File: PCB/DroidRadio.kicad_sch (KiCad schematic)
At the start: 31 parts, among them T1 MABA-007159, U1 LTC5599IUF, U2 ADF4351

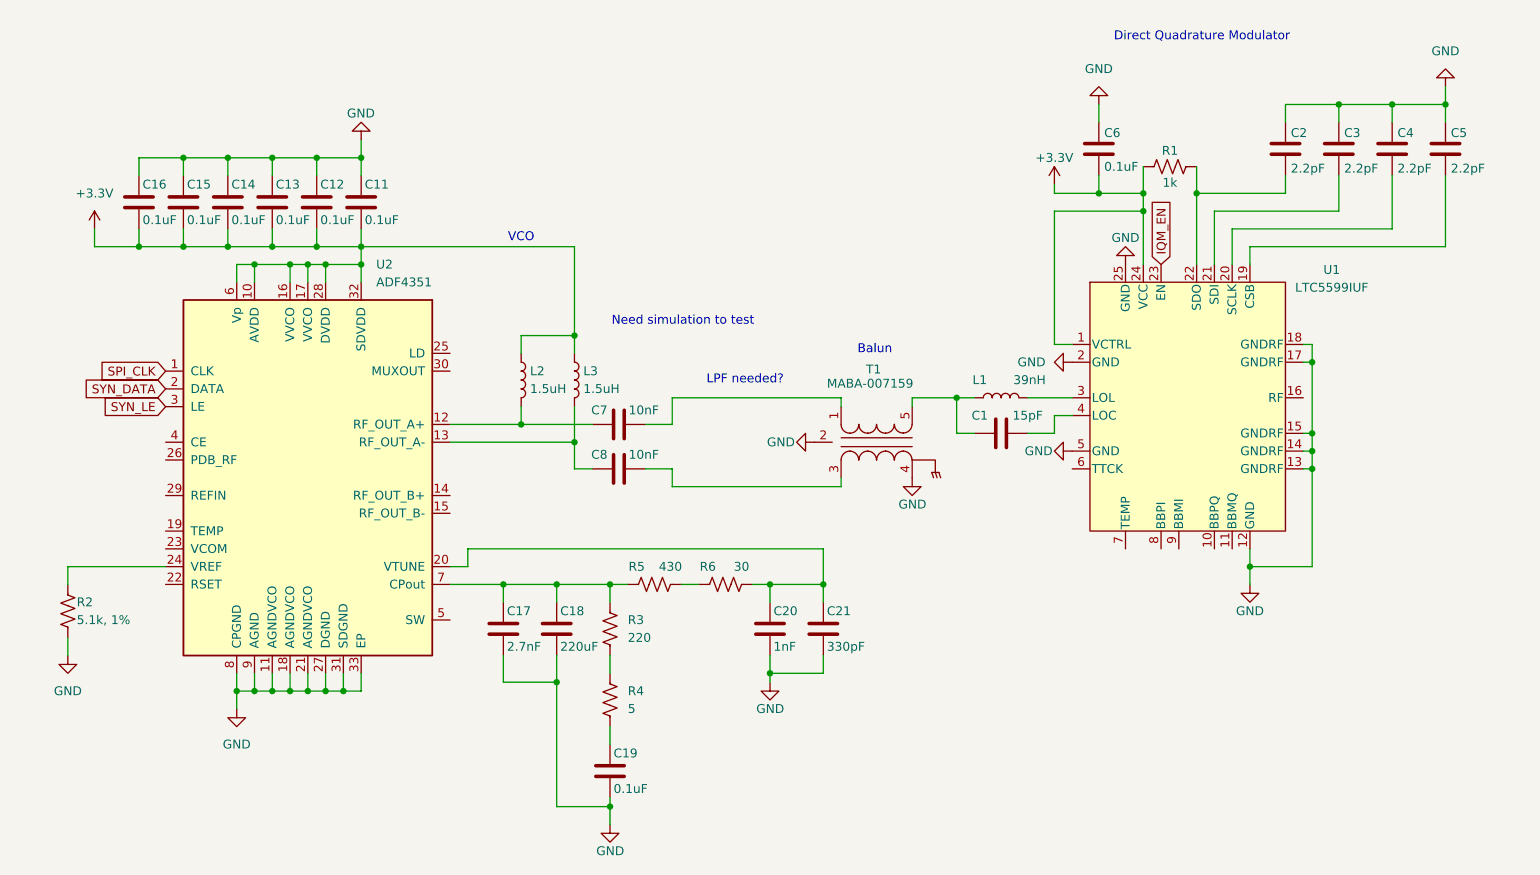
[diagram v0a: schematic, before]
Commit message: new file:   .gitignore 	modified:   PCB/DroidRadio.kicad_pro 	modified:   PCB/DroidRadio.kicad_sch 	new file:   PCB/Processors.kicad_sch 	new file:   PCB/Transmitter.kicad_sch 	deleted:    PCB/_autosave-Transmitter.kicad_sch 	new file:   PCB/~DroidRadio.kicad_pro.lck
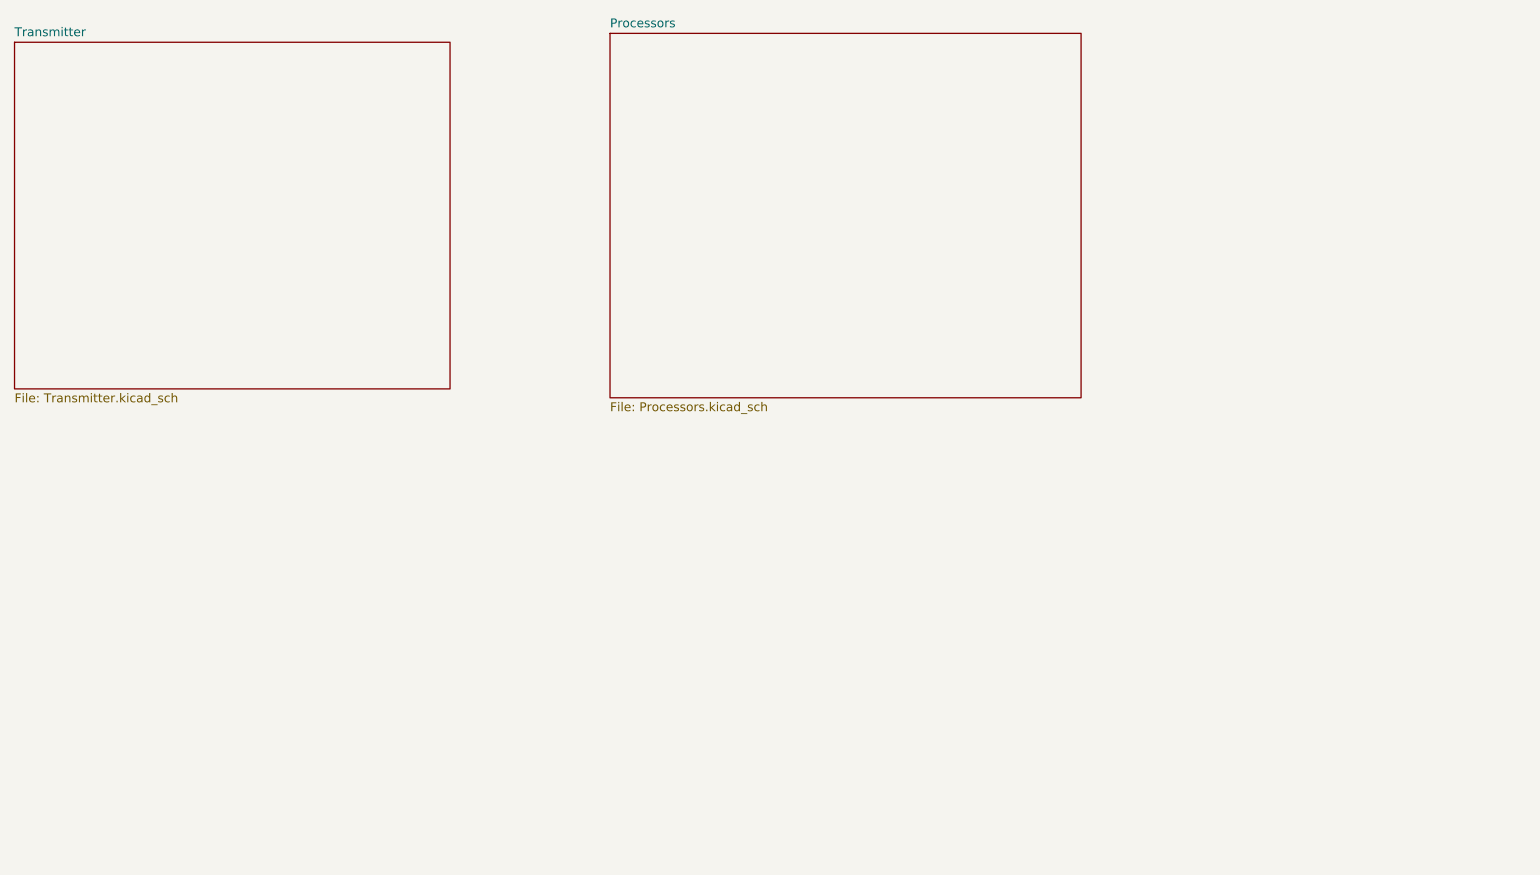
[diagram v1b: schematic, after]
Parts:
- removed C1: 15pF, symbol Device:C
- removed C11, C12, C13, C14, C15, C16, C19, C6: 0.1uF, symbol Device:C
- removed C17: 2.7nF, symbol Device:C
- removed C18: 220uF, symbol Device:C
- removed C2, C3, C4, C5: 2.2pF, symbol Device:C
- removed C20: 1nF, symbol Device:C
- removed C21: 330pF, symbol Device:C
- removed C7, C8: 10nF, symbol Device:C
- removed L1: 39nH, symbol Device:L
- removed L2, L3: 1.5uH, symbol Device:L
- removed R1: 1k, symbol Device:R_US
- removed R2: 5.1k, 1%, symbol Device:R_US
- removed R3: 220, symbol Device:R_US
- removed R4: 5, symbol Device:R_US
- removed R5: 430, symbol Device:R_US
- removed R6: 30, symbol Device:R_US
- removed T1: MABA-007159, MABA-007159-000000_MCM, symbol DroidRadio:MABA-007159
- removed U1: LTC5599IUF, DroidRadio:QFN-24_UF_LIT, symbol DroidRadio:LTC5599IUF
- removed U2: ADF4351, Package_CSP:LFCSP-32-1EP_5x5mm_P0.5mm_EP3.25x3.25mm, symbol Timer_PLL:ADF4351
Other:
- added sheet Processors (Processors.kicad_sch)
- added sheet Transmitter (Transmitter.kicad_sch)
- note removed: "Balun"
- note removed: "Direct Quadrature Modulator"
- note removed: "LPF needed?"
- note removed: "Need simulation to test"
- note removed: "VCO"

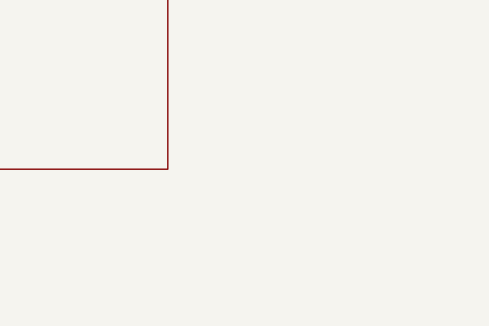
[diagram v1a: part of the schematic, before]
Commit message: new file:   Datasheet/HMC849A_RF_Switch_SPDT.pdf 	new file:   Datasheet/TG2016SMN_26MHz_MCGNNM_Oscillator.pdf 	modified:   PCB/DroidRadio.kicad_pro 	modified:   PCB/DroidRadio.kicad_sch 	modified:   PCB/Processors.kicad_sch 	modified:   PCB/Simulation/Transmitter_Side.pll 	modified:   PCB/Transmitter.kicad_sch 	deleted:    PCB/~DroidRadio.kicad_pro.lck
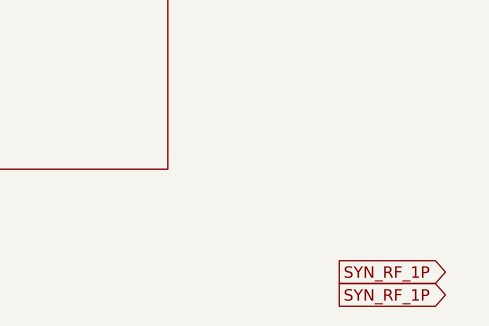
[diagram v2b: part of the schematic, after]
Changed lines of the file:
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@@
 	(generator_version "10.0")
 	(paper "A4")
+	(global_label "SYN_RF_1P"
+		(shape output)
+		(at 205.74 96.52 0)
+		(fields_autoplaced yes)
+		(effects
+			(font
+				(size 1.27 1.27)
+			)
+			(justify left)
+		)
+		(property "Intersheetrefs" "${INTERSHEET_REFS}"
+			(at 219.1271 96.52 0)
+			(hide yes)
+			(show_name no)
+			(do_not_autoplace no)
+			(effects
+				(font
+					(size 1.27 1.27)
+				)
+				(justify left)
+			)
+		)
+	)
+	(global_label "SYN_RF_1P"
+		(shape output)
+		(at 205.74 99.06 0)
+		(fields_autoplaced yes)
+		(effects
+			(font
+				(size 1.27 1.27)
+			)
+			(justify left)
+		)
+		(property "Intersheetrefs" "${INTERSHEET_REFS}"
+			(at 219.1271 99.06 0)
+			(hide yes)
+			(show_name no)
+			(do_not_autoplace no)
+			(effects
+				(font
+					(size 1.27 1.27)
+				)
+				(justify left)
+			)
+		)
+	)
 	(sheet
 		(at 34.29 34.29)

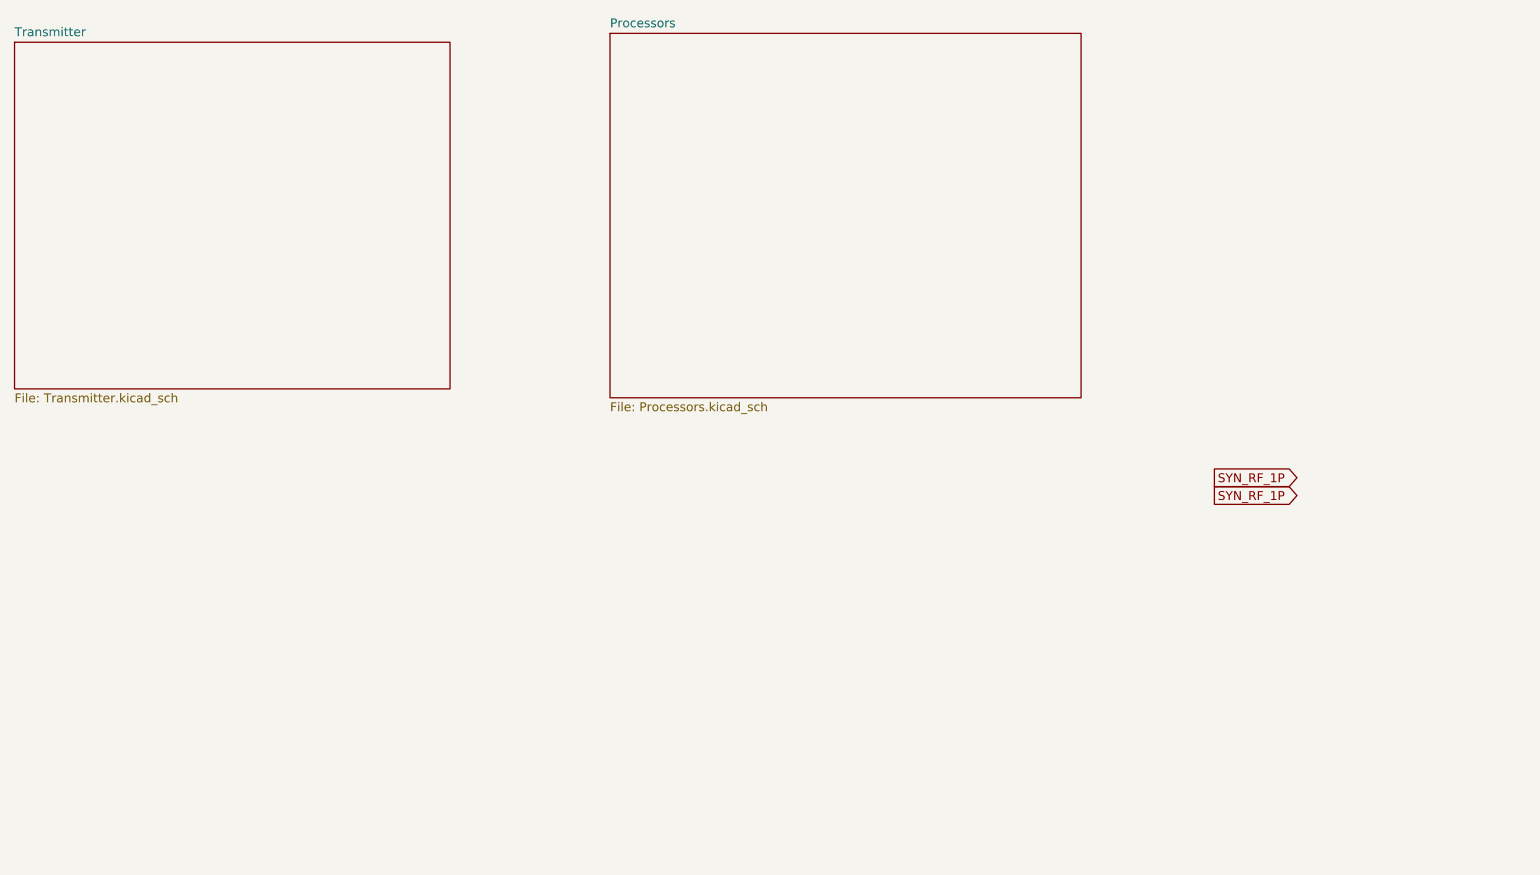
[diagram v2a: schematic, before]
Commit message: Updated PCB schematics, added new datasheet and components library
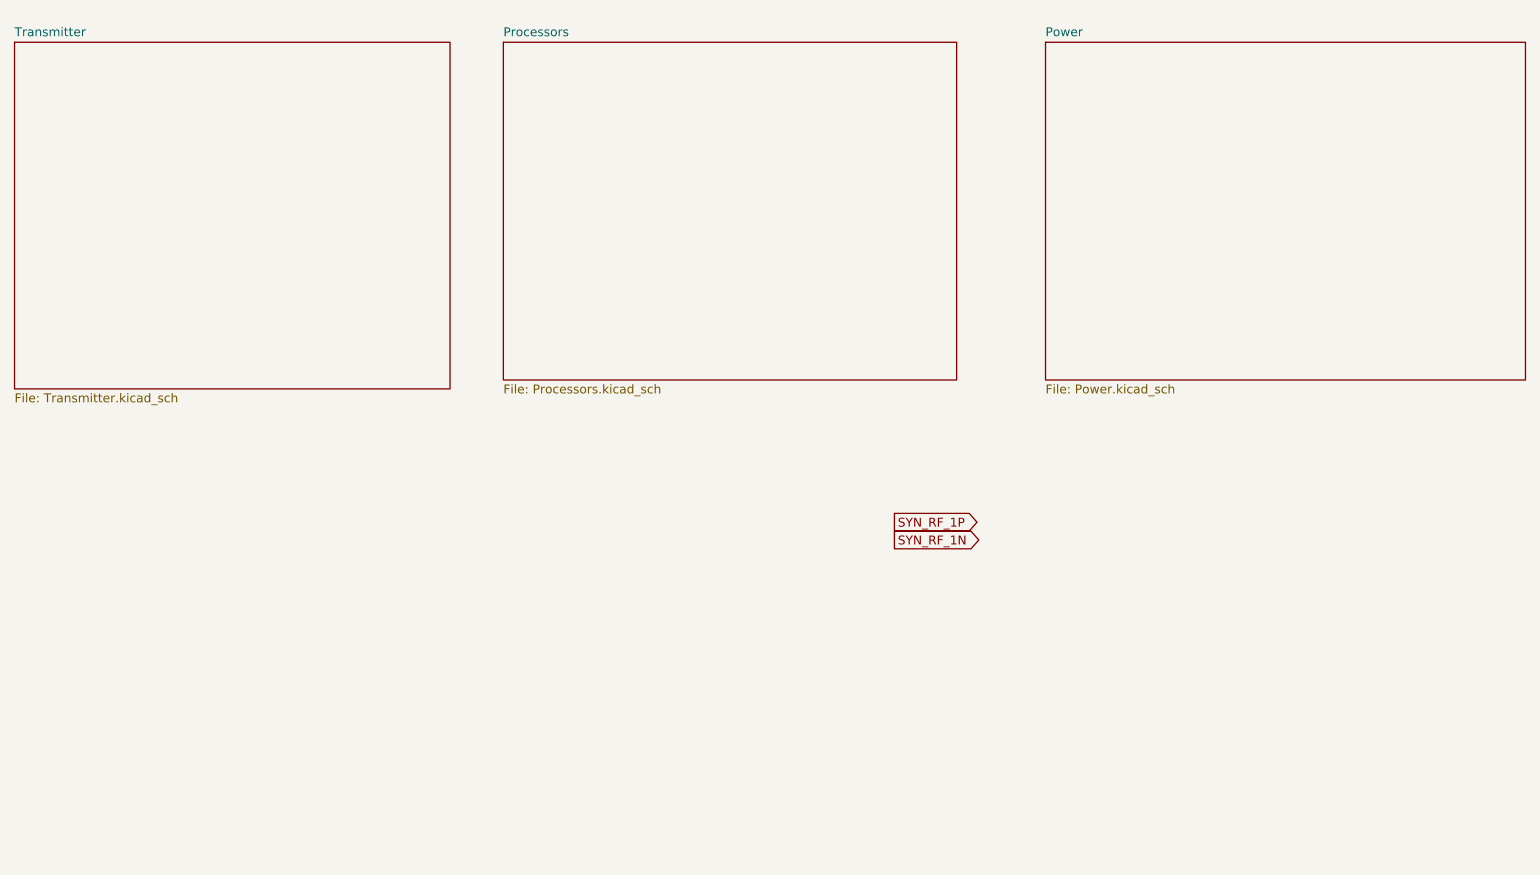
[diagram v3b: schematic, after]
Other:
- added sheet Power (Power.kicad_sch)
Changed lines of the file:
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@@
 	(generator_version "10.0")
 	(paper "A4")
-	(global_label "SYN_RF_1P"
+	(global_label "SYN_RF_1N"
 		(shape output)
-		(at 205.74 96.52 0)
+		(at 160.02 105.41 0)
 		(fields_autoplaced yes)
 		(effects
@@
 		)
 		(property "Intersheetrefs" "${INTERSHEET_REFS}"
-			(at 219.1271 96.52 0)
+			(at 173.4676 105.41 0)
 			(hide yes)
 			(show_name no)
@@
 	(global_label "SYN_RF_1P"
 		(shape output)
-		(at 205.74 99.06 0)
+		(at 160.02 102.87 0)
 		(fields_autoplaced yes)
 		(effects
@@
 		)
 		(property "Intersheetrefs" "${INTERSHEET_REFS}"
-			(at 219.1271 99.06 0)
+			(at 173.4071 102.87 0)
 			(hide yes)
 			(show_name no)
@@
 	)
 	(sheet
-		(at 119.38 33.02)
-		(size 67.31 52.07)
+		(at 181.61 34.29)
+		(size 68.58 48.26)
+		(exclude_from_sim no)
+		(in_bom yes)
+		(on_board yes)
+		(dnp no)
+		(fields_autoplaced yes)
+		(stroke
+			(width 0.1524)
+			(type solid)
+		)
+		(fill
+			(color 0 0 0 0)
+		)
+		(property "Sheetname" "Power"
+			(at 181.61 33.5784 0)
+			(show_name no)
+			(do_not_autoplace no)
+			(effects
+				(font
+					(size 1.27 1.27)
+				)
+				(justify left bottom)
+			)
+		)
+		(property "Sheetfile" "Power.kicad_sch"
+			(at 181.61 83.1346 0)
+			(show_name no)
+			(do_not_autoplace no)
+			(effects
+				(font
+					(size 1.27 1.27)
+				)
+				(justify left top)
+			)
+		)
+		(instances
+			(project "DroidRadio"
+				(path "/b5ecdb3b-a3b2-44a8-986c-aaad7cd56a32"
+					(page "4")
+				)
+			)
+		)
+	)
+	(sheet
+		(at 104.14 34.29)
+		(size 64.77 48.26)
 		(exclude_from_sim no)
 		(in_bom yes)
@@
 		)
 		(property "Sheetname" "Processors"
-			(at 119.38 32.3084 0)
+			(at 104.14 33.5784 0)
 			(show_name no)
 			(do_not_autoplace no)
@@
 		)
 		(property "Sheetfile" "Processors.kicad_sch"
-			(at 119.38 85.6746 0)
+			(at 104.14 83.1346 0)
 			(show_name no)
 			(do_not_autoplace no)
